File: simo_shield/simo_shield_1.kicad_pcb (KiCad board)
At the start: 2 copper layers, 70 x 100 mm, 10 parts, among them J1 Conn_01x02_Female, J2 Conn_01x02_Female, U1 elemon_board, U2 modulo_flash_externa, U3 bluepill_board_stm32, U4 modulo_acelerometro

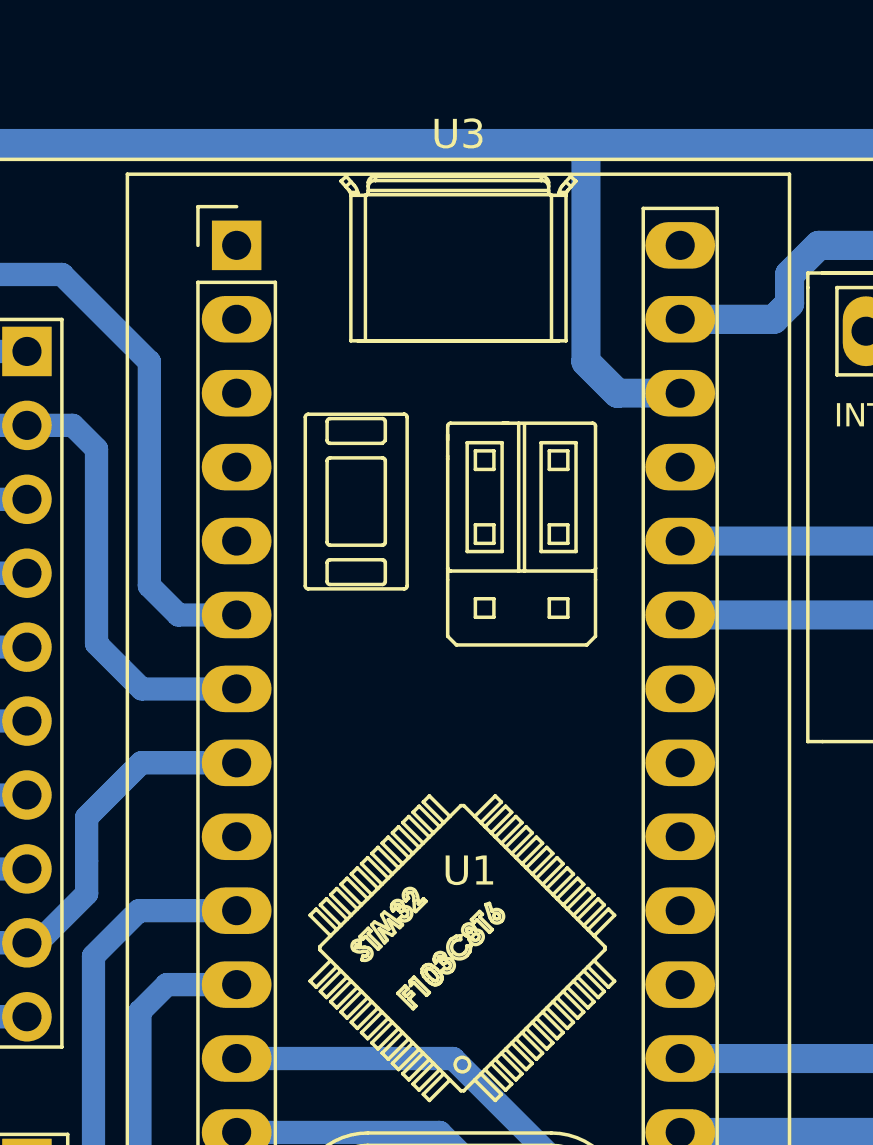
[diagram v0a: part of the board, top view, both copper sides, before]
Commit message: actualizaciones a pcb y esquema simo shield
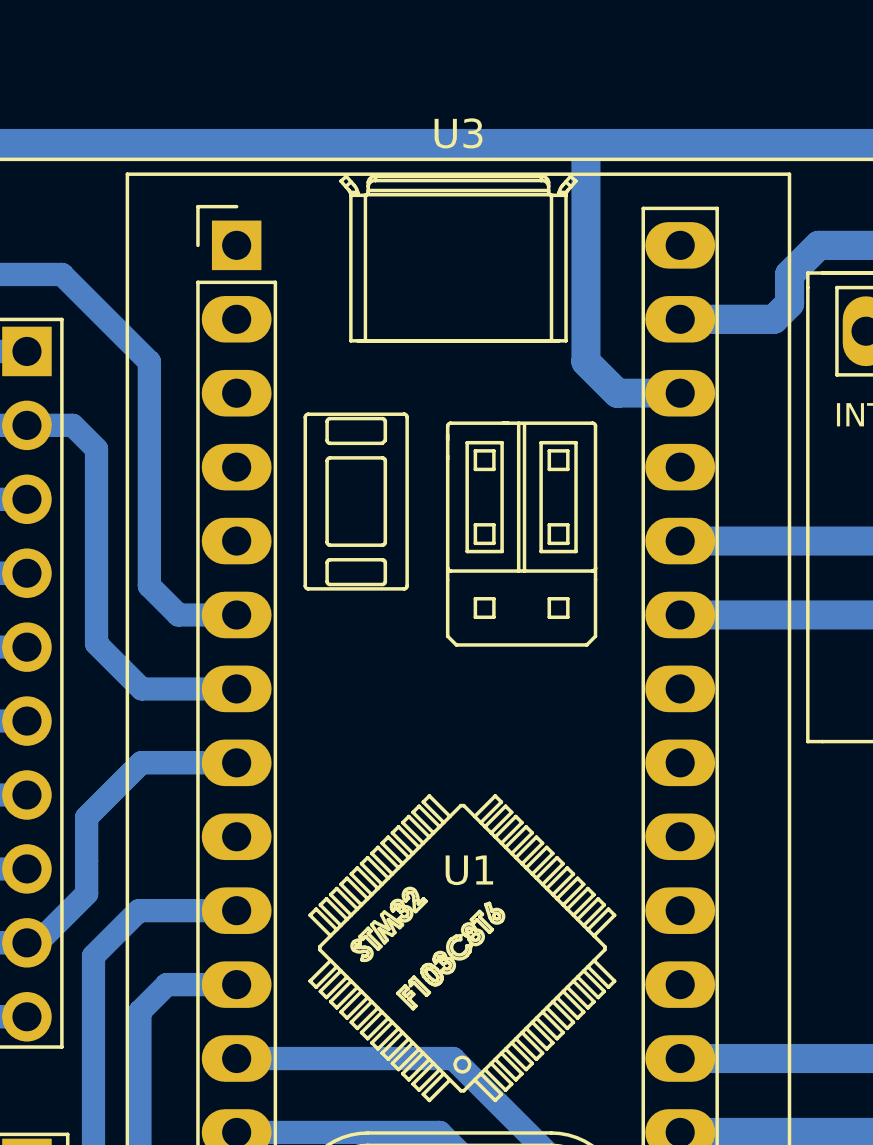
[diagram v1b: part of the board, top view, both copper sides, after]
